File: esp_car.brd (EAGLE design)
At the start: 81.6 x 84 mm, 50 parts, among them IC2 LT1963ES8-3.3, SW2 SK-12D01, U1 ESP-WROOM-32_NOFLASH

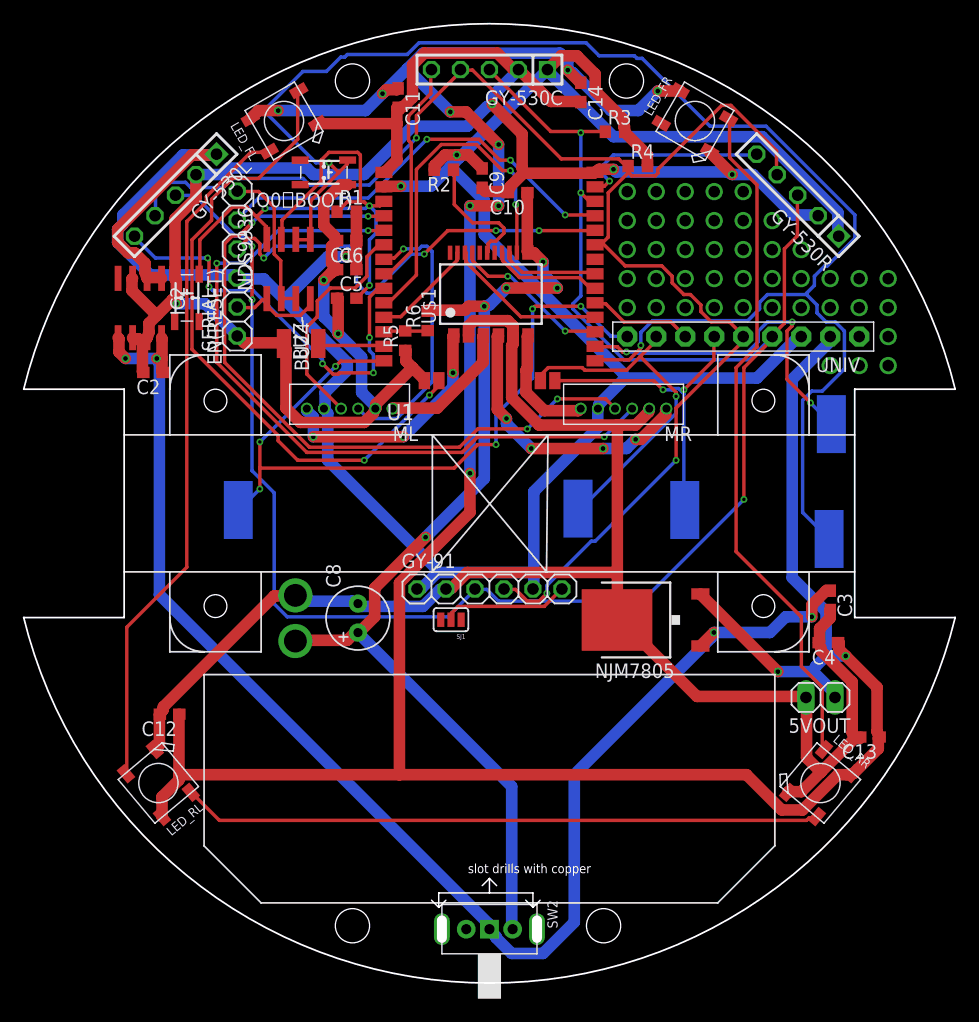
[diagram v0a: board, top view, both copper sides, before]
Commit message: wire 100% 初版
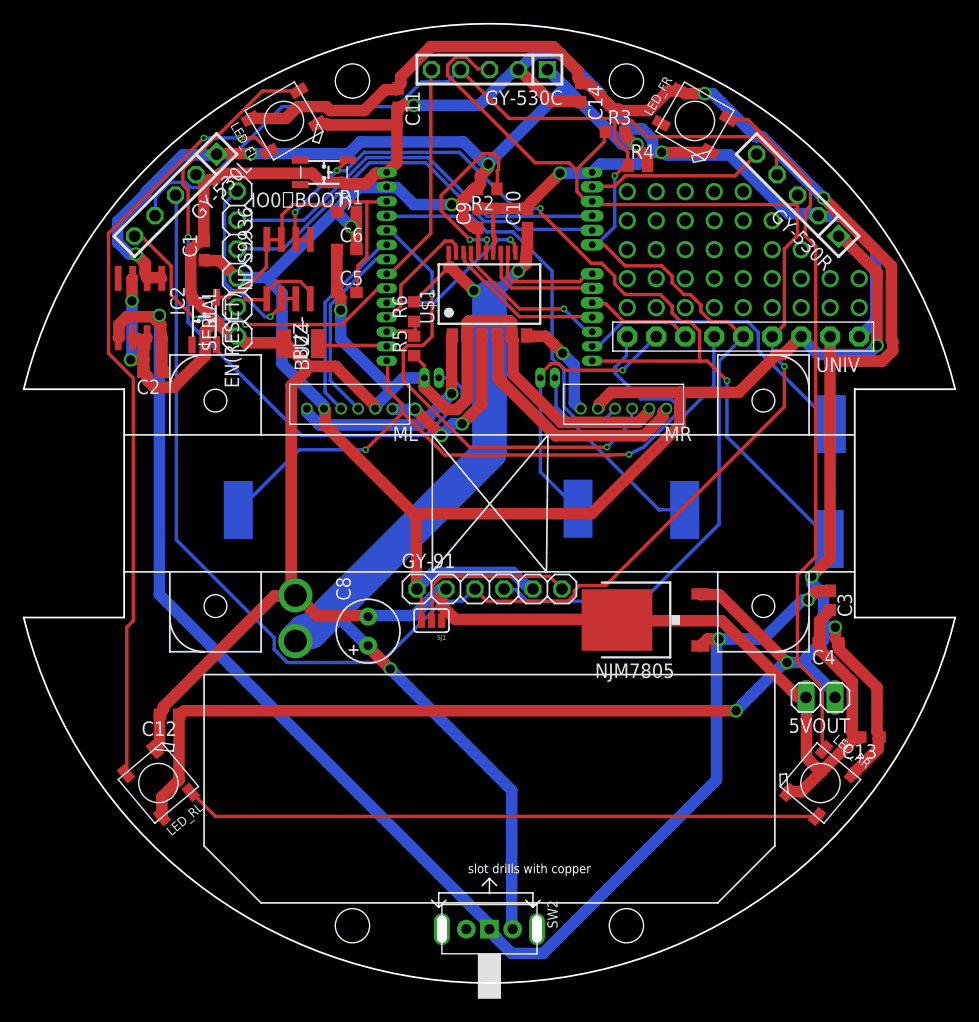
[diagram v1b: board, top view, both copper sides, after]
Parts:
- removed U1: ESP-WROOM-32_NOFLASH, esp32 _my:ESP-WROOM-32_NOFLASH
- added ESP32: ESP-WROOM-32_NOFLASH_PINHEAD, esp32 _my:ESP-WROOM-32_NOFLASH_PINHEAD
- moved C1 12.5 mm to (15.0, 62.2), turned to 90 degrees
- moved R2 4.15 mm to (39.8, 67.6)
- moved C9 3.53 mm to (39.0, 65.0), turned to 90 degrees
- moved EN(RESET) 2.54 mm to (15.0, 56.0)
- moved C10 2.42 mm to (43.3, 65.0), turned to 90 degrees
- moved C6 1.78 mm to (27.5, 62.2)
- moved SJ1 1.70 mm to (34.9, 29.7)
- moved C8 1.45 mm to (29.4, 28.8)
- moved R6 1.44 mm to (33.4, 56.8)
- moved R5 0.90 mm to (33.4, 53.8)
- moved C5 0.51 mm to (27.5, 58.5)
- moved U$1 0.13 mm to (40.0, 58.3)
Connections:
- net +3V3: now also ESP32.P$2; no longer U1.2
- net EN: now also ESP32.P$3; no longer U1.3
- net ENCL_A: now also ESP32.P$6; no longer U1.6
- net ENCL_B: now also ESP32.P$7; no longer U1.7
- net ENCR_A: now also ESP32.P$4; no longer U1.4
- net ENCR_B: now also ESP32.P$5; no longer U1.5
- net GND: now also ESP32.P$1, ESP32.P$15, ESP32.P$38; no longer U1.1, U1.15, U1.38
- net I2C_SCL: now also ESP32.P$36; no longer U1.36
- net I2C_SDA: now also ESP32.P$33; no longer U1.33
- net IO0: now also ESP32.P$25; no longer U1.25
- net IO12: now also ESP32.P$14; no longer U1.14
- net IO15: now also ESP32.P$23; no longer U1.23
- net IO2: now also ESP32.P$24; no longer U1.24
- net IO27: now also ESP32.P$12; no longer U1.12
- net IO4: now also ESP32.P$26; no longer U1.26
- net IO5: now also ESP32.P$29; no longer U1.29
- net ML_IN1: now also ESP32.P$27; no longer U1.27
- net ML_IN2: now also ESP32.P$28; no longer U1.28
- net ML_PWM: now also ESP32.P$11; no longer U1.11
- net MR_IN1: now also ESP32.P$30; no longer U1.30
- net MR_IN2: now also ESP32.P$31; no longer U1.31
- net MR_PWM: now also ESP32.P$10; no longer U1.10
- net N$18: now also ESP32.P$16; no longer U1.16
- net N$19: now also ESP32.P$9; no longer U1.9
- net N$3: now also ESP32.P$8; no longer U1.8
- net N$5: now also ESP32.P$37; no longer U1.37
- net N$8: now also ESP32.P$13; no longer U1.13
- net RX: now also ESP32.P$34; no longer U1.34
- net TX: now also ESP32.P$35; no longer U1.35
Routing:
- net IO0: track 135.8 -> 82.8 mm, vias 2 -> 4
- net +5V: track 252.5 -> 209.7 mm, vias 11 -> 6
- net ENCR_A: track 64.8 -> 34.2 mm, vias 4 -> 0
- net ENCR_B: track 65.8 -> 41.5 mm, vias 3 -> 2
- net EN: track 52.3 -> 29.9 mm, vias 3 -> 0
- net GND: track 335.2 -> 357.0 mm
- net MR_PWM: track 30.6 -> 14.4 mm, vias 2 -> 1
- net +3V3: track 238.8 -> 226.0 mm, vias 3 -> 7
- net N$19: track 36.0 -> 28.2 mm, vias 5 -> 2
- net ENCL_B: track 24.5 -> 16.7 mm, vias 1 -> 0
- net N$6: track 60.7 -> 66.5 mm, vias 0 -> 2
- net N$7: track 11.3 -> 17.0 mm, vias 0 -> 2
- net IO15: track 30.7 -> 25.2 mm
- net IO2: track 28.1 -> 33.0 mm, vias 2 -> 0
- net VCC: track 124.3 -> 128.8 mm, vias 4 -> 3
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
